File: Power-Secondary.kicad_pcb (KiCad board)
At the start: 2 copper layers, 116 x 67 mm, 32 parts, among them J1 SUPP PWR, J2 DCDC SUPPLY, J3 JUMP START, J4 FUSE +12V, Q1 AUIRF4905, SW1 SUPP PWR CHECK, SW2 FUSE PWR CHECK

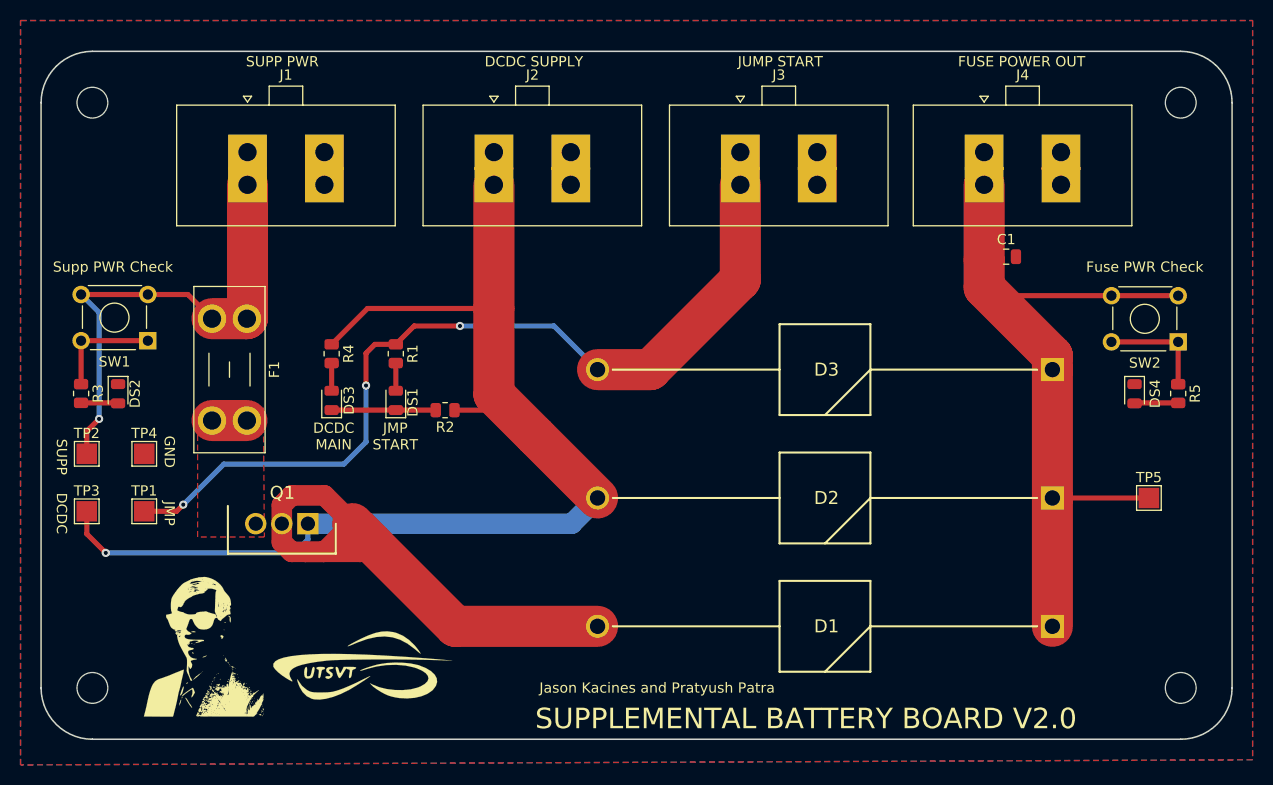
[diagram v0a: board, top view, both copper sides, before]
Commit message: version 3
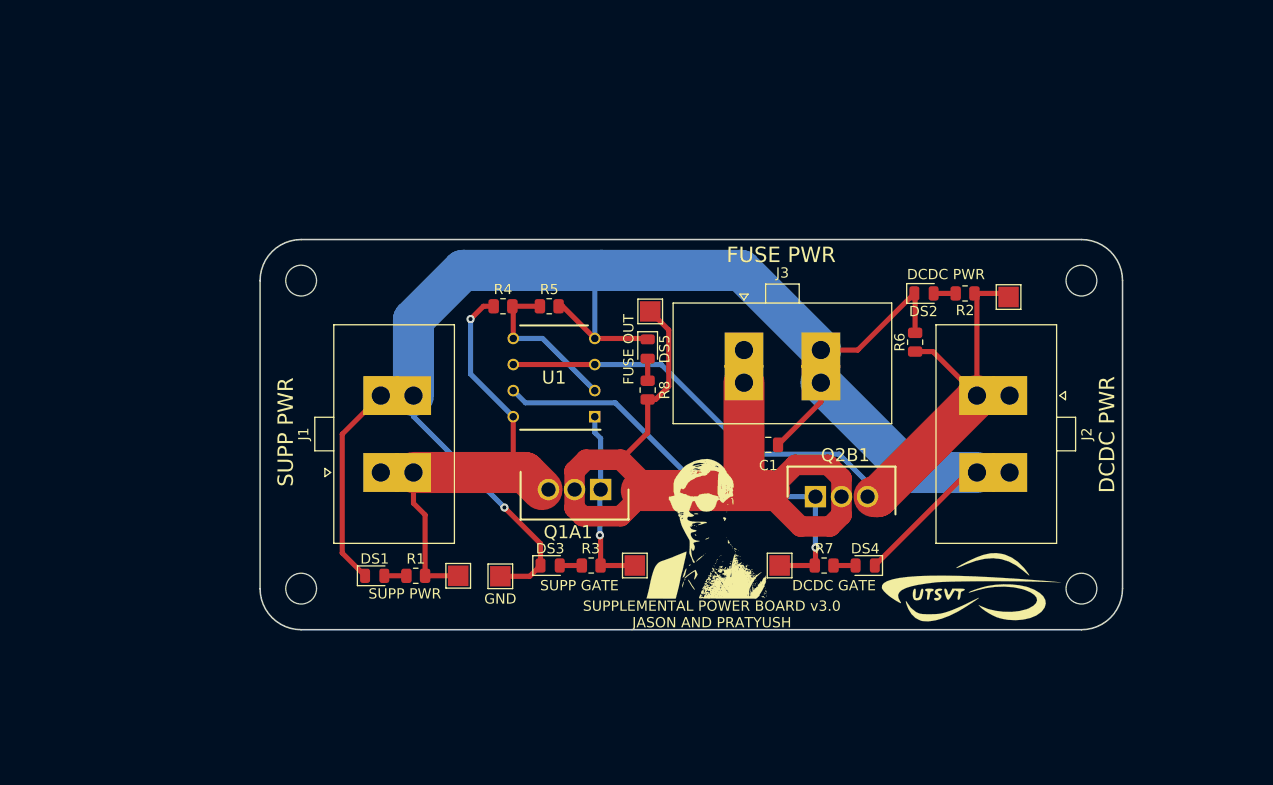
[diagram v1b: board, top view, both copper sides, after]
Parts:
- removed D1, D2, D3: V25PN60, UTSVT_PowerSupp:DIOAD4425W130L885D885
- removed F1: 20 AMPS, Fuse:Fuseholder_Blade_Mini_Keystone_3568
- removed J4: FUSE +12V, Connector_Molex:Molex_Sabre_43160-0102_1x02_P7.49mm_Vertical
- removed Q1: AUIRF4905, UTSVT_PowerSupp:TO254P465X1031X1954-3P
- removed SW1: SUPP PWR CHECK, Button_Switch_THT:SW_TH_Tactile_Omron_B3F-10xx
- removed SW2: FUSE PWR CHECK, Button_Switch_THT:SW_TH_Tactile_Omron_B3F-10xx
- added DS5: FUSE_OUT, Diode_SMD:D_0805_2012Metric, F.Cu at (146.1, 97.0)
- added Q1A1: SUP90P06-PCHANNEL-MOSFET, UTSVT_PowerSupp:SUP90P06-PCHAN-ENH-PWR-MOSFET, F.Cu at (141.5, 110.7)
- added Q2B1: SUP90P06-PCHANNEL-MOSFET, UTSVT_PowerSupp:SUP90P06-PCHAN-ENH-PWR-MOSFET, F.Cu at (162.4, 111.4)
- added R6: 100K, Resistor_SMD:R_0805_2012Metric, F.Cu at (172.1, 96.3)
- added R7: 5.1K, Resistor_SMD:R_0805_2012Metric, F.Cu at (163.3, 118.1)
- added R8: 5.1K, Resistor_SMD:R_0805_2012Metric, F.Cu at (146.1, 101.0)
- added TP6: GND, TestPoint:TestPoint_Pad_2.0x2.0mm, F.Cu at (131.7, 119.1)
- added U1: Opamp_Dual, UTSVT_PowerSupp:LM358P-OPAMP, F.Cu at (137.0, 99.8)
- DS1: value JUMP START ON -> SUPP_PWR
- DS2: value SUPP PWR -> DCDC_PWR
- DS3: value DCDC MAIN SUPPLY ON -> SUPP_GATE
- DS4: value FUSE PWR -> DCDC_GATE
- J3: value JUMP START -> FUSE +12V
- R2: value 100k -> 5.1K
- R4: value 5.1K -> 10K
- R5: value 5.1K -> 180K
- TP1: value JUMP START VOLTS -> SUPP_PWR
- TP2: value SUPP SUPPLY VOLTS -> DCDC_PWR
- TP3: value DCDC MAIN SUPPLY -> SUPP_GATE
- TP4: value GND -> DCDC_GATE
- TP5: value FUSE SUPPLY VOLTS -> FUSE_OUT
- moved TP2 91.1 mm to (181.2, 91.9)
- moved DS2 79.1 mm to (173.0, 91.6), turned to 0 degrees
- moved TP4 62.8 mm to (158.9, 118.1)
- moved R5 61.8 mm to (136.5, 92.8), turned to 0 degrees
- moved LOGO2 59.8 mm to (177.3, 120.3)
- moved TP3 53.6 mm to (144.8, 118.1)
- moved R3 52.4 mm to (140.6, 118.1), turned to 180 degrees
- moved R2 51.9 mm to (177.0, 91.6)
- moved TP5 51.9 mm to (146.3, 93.3)
- moved J2 51.3 mm to (178.2, 101.5), turned to -90 degrees
- moved LOGO1 50.3 mm to (151.3, 114.3)
- moved J1 32.3 mm to (123.3, 109.0), turned to 90 degrees
- moved TP1 31.2 mm to (127.6, 119.1)
- moved DS4 31.1 mm to (167.3, 118.1), turned to 180 degrees
- moved C1 29.5 mm to (157.8, 106.3)
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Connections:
- C1 pad 1: Net-(C1-Pad1) -> FUSE_OUT
- J1 pad 1: Net-(F1-Pad1) -> SUPP_PWR
- J2 pad 1: Net-(D2-Pad2) -> DCDC_PWR
- J3 pad 1: Net-(D3-Pad2) -> FUSE_OUT
- R1 pad 1: Net-(D3-Pad2) -> SUPP_PWR
- R2 pad 1: Net-(D2-Pad2) -> DCDC_PWR
- R2 pad 2: GNDS -> Net-(DS2-Pad2)
- R3 pad 1: Net-(R3-Pad1) -> SUPP_GATE
- R3 pad 2: Net-(DS2-Pad2) -> Net-(DS3-Pad2)
- R4 pad 1: Net-(D2-Pad2) -> SUPP_PWR
- R4 pad 2: Net-(DS3-Pad2) -> V_REF
- R5 pad 1: Net-(R5-Pad1) -> V_REF
- R5 pad 2: Net-(DS4-Pad2) -> GNDS
- TP1 pad 1: Net-(D3-Pad2) -> SUPP_PWR
- TP2 pad 1: Net-(F1-Pad1) -> DCDC_PWR
- TP3 pad 1: Net-(D2-Pad2) -> SUPP_GATE
- TP4 pad 1: GNDS -> DCDC_GATE
- TP5 pad 1: Net-(C1-Pad1) -> FUSE_OUT
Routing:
- net GNDS: track 10.1 -> 170.8 mm, vias 0 -> 1
- net Net-(D2-Pad2): track 116.7 -> 0.00 mm, vias 1 -> 0
- net Net-(D3-Pad2): track 85.2 -> 0.00 mm, vias 3 -> 0
- net FUSE_OUT: track 0.00 -> 83.9 mm
- net DCDC_PWR: track 0.00 -> 76.2 mm
- net Net-(C1-Pad1): track 75.3 -> 0.00 mm
- net Net-(D1-Pad2): track 55.2 -> 0.00 mm
- net Net-(F1-Pad1): track 46.9 -> 0.00 mm, vias 1 -> 0
- net SUPP_PWR: track 0.00 -> 46.9 mm, vias 0 -> 1
- net DCDC_GATE: track 0.00 -> 43.9 mm, vias 0 -> 1
- net SUPP_GATE: track 0.00 -> 18.1 mm, vias 0 -> 1
- net V_REF: track 0.00 -> 15.9 mm
- net Net-(R3-Pad1): track 10.7 -> 0.00 mm
- net Net-(R5-Pad1): track 10.6 -> 0.00 mm
- net Net-(F1-Pad2): track 3.40 -> 0.00 mm
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- removed copper zone on B.Cu, net GNDS
- removed copper zone on F.Cu, net GNDS
- removed copper zone on F.Cu, net Net-(F1-Pad2)
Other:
- board size 116 x 67 mm -> 84 x 38 mm
- board text added: "DCDC GATE"
- board text added: "DCDC PWR"
- board text added: "FUSE OUT"
- board text added: "FUSE PWR"
- board text added: "SUPP GATE"
- board text added: "SUPPLEMENTAL POWER BOARD v3.0 JASON AND PRATYUSH"
- board text removed: "DCDC"
- board text removed: "DCDC MAIN"
- board text removed: "DCDC SUPPLY"
- board text removed: "FUSE POWER OUT"
- board text removed: "Fuse PWR Check"
- board text removed: "JMP"
- board text removed: "JMP START"
- board text removed: "JUMP START"
- board text removed: "Jason Kacines and Pratyush Patra"
- board text removed: "SUPP"
- board text removed: "SUPPLEMENTAL BATTERY BOARD V2.0"
- board text removed: "Supp PWR Check"
